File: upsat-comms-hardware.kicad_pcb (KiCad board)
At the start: 4 copper layers, 92.5 x 92.5 mm, 313 parts, among them U1 TXCO_TG_5021CG, U10 CC1120, U12 ADT7420, U14 OPA320, U16 RF5110G, U18 FA_128_, U2 TPS79930, U3 FA_128_, U4 CC1120, U5 STM32F407VG, U6 TXCO_TG_5021CG, U8 TPS79930, Y1 Crystal, Y2 Crystal

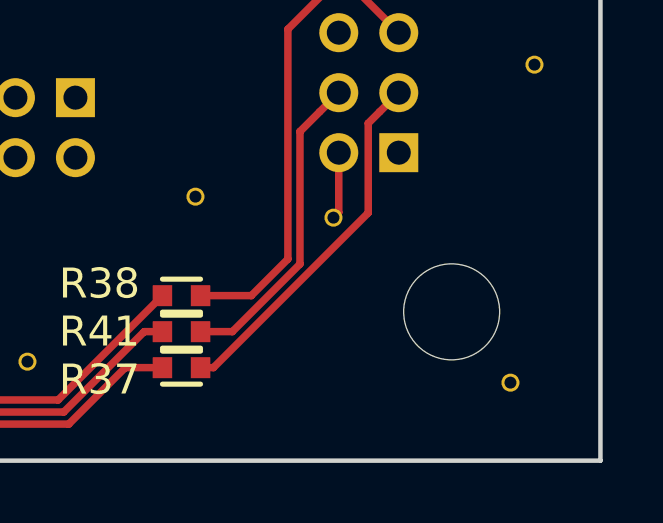
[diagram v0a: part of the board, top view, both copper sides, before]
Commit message: Fixed small mistake
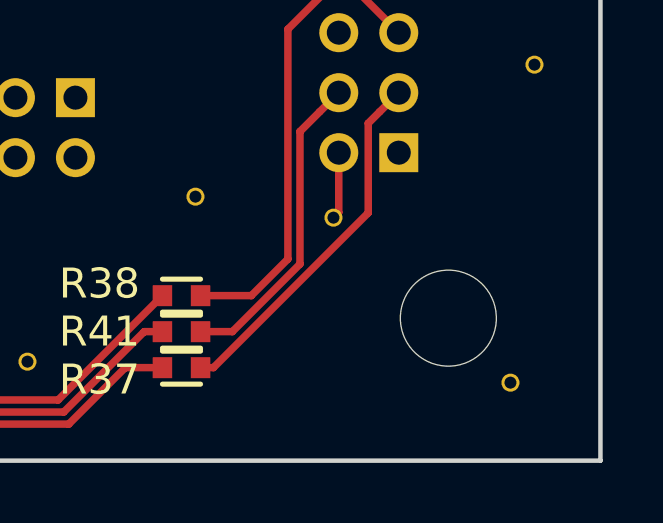
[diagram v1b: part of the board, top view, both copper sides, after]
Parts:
- moved REF** 0.24 mm to (189.9, 142.3)
